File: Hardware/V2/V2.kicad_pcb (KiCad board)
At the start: 2 copper layers, 115 x 61 mm, 69 parts, among them J1 USB_B_Mini, J2 I2C_OLED, J3 ICSP, J4 BT_CONN, J5 BAT, Q1 MMBT2222, SW1 SW_Push, SW2 SW_Push, SW3 SW_Push, U1 ATmega32U4-AU, U2 LIS3DH, U3 DHT11, U4 AP2112K-3.3, Y1 16MHz

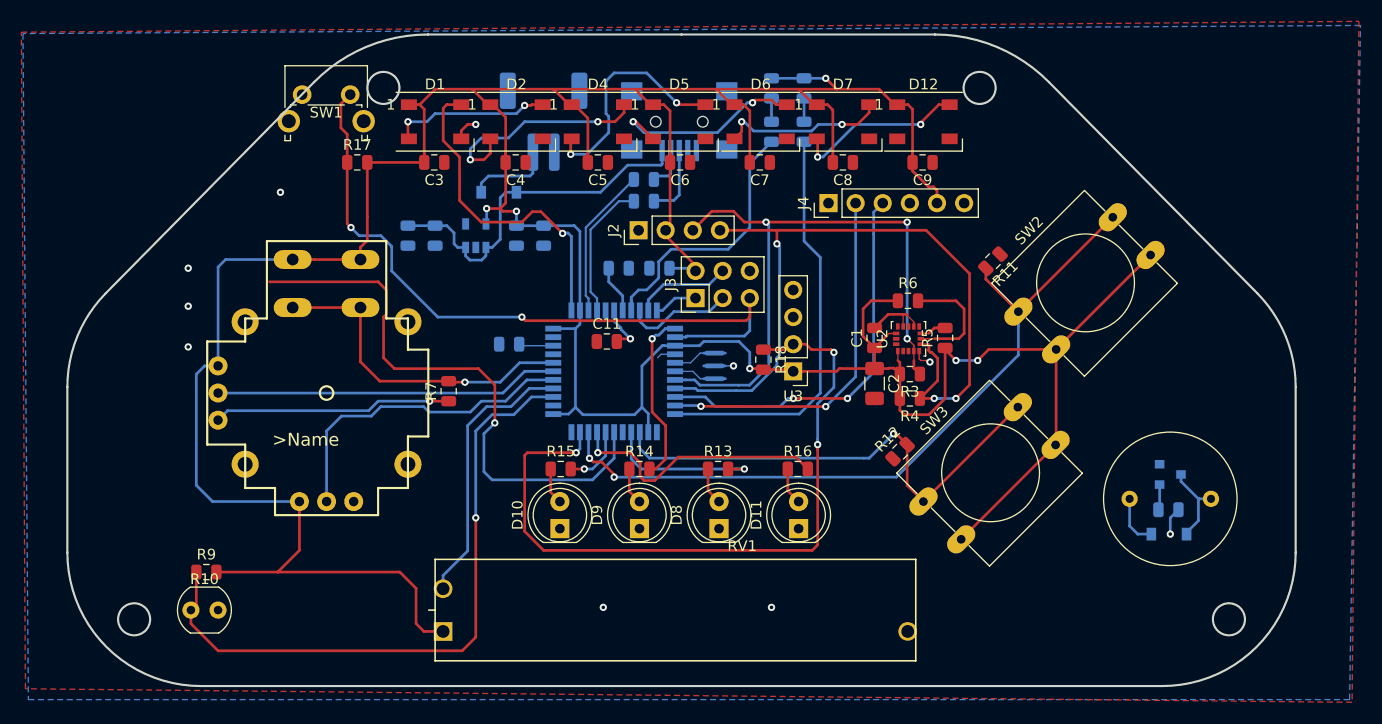
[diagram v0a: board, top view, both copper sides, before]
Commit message: Placa enrutada
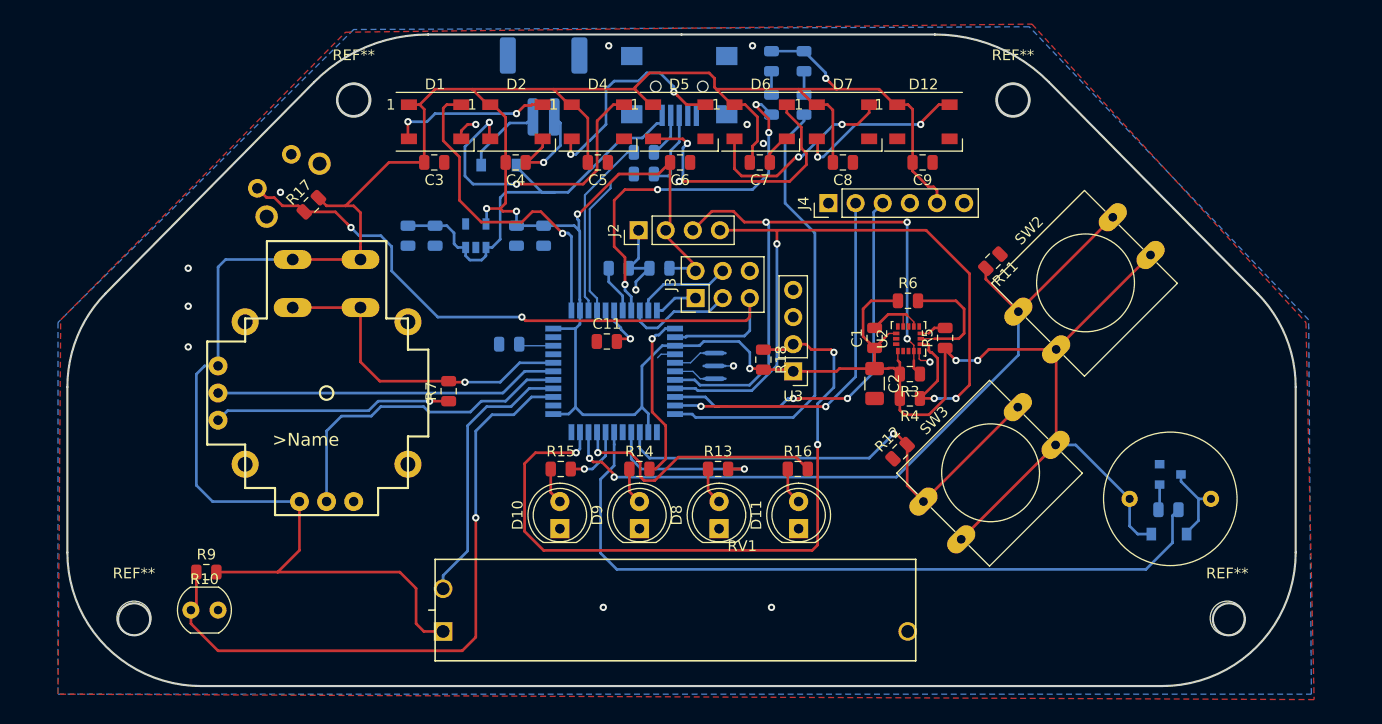
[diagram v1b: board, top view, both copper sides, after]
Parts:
- added REF**: MountingHole_3.2mm_M3, MountingHole:MountingHole_3.2mm_M3, F.Cu at (125.7, 61.5)
- added REF**: MountingHole_3.2mm_M3, MountingHole:MountingHole_3.2mm_M3, F.Cu at (187.5, 61.5)
- added REF**: MountingHole_3.2mm_M3, MountingHole:MountingHole_3.2mm_M3, F.Cu at (207.5, 110.0)
- added REF**: MountingHole_3.2mm_M3, MountingHole:MountingHole_3.2mm_M3, F.Cu at (105.2, 110.0)
- SW1: moved to B.Cu
- moved R17 5.85 mm to (121.8, 71.3), turned to 45 degrees
- moved SW1 5.68 mm to (119.9, 66.5), turned to 225 degrees
- moved J1 3.30 mm to (156.2, 60.2)
- moved J5 3.30 mm to (143.5, 60.2)
- moved D15 2.54 mm to (139.3, 67.6)
- moved R1 2.54 mm to (152.9, 68.4)
- moved R2 2.54 mm to (152.9, 66.4)
- moved D13 2.54 mm to (164.8, 57.8)
- moved D14 2.54 mm to (167.9, 57.8)
- moved R19 2.54 mm to (164.8, 61.9)
- moved R20 2.54 mm to (167.9, 61.9)
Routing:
- net +3V3: track 378.2 -> 400.7 mm, vias 6 -> 7
- net GND: track 36.4 -> 58.0 mm, vias 10 -> 16
- net BUZZ: track 56.1 -> 70.4 mm, vias 2 -> 0
- net Net-(R19-Pad2): track 25.8 -> 35.3 mm, vias 0 -> 4
- net Net-(D2-Pad2): track 21.0 -> 28.5 mm
- net Net-(D5-Pad2): track 18.8 -> 26.2 mm
- net VUSB: track 33.9 -> 38.9 mm
- net Net-(R20-Pad2): track 38.6 -> 42.3 mm
- net Net-(D6-Pad2): track 15.6 -> 19.2 mm
- net D-: track 14.2 -> 17.2 mm
- net D+: track 13.0 -> 15.6 mm
- net RST: track 67.7 -> 65.3 mm
- net Net-(D4-Pad2): track 21.7 -> 20.7 mm
- net Net-(D15-Pad2): track 8.04 -> 7.46 mm
- net Net-(J1-Pad2): track 3.96 -> 3.43 mm
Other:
- outline, holes or cut-outs redrawn
